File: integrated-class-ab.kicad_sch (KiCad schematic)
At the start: 31 parts, among them J1001 LABEL, Q1001 MMBT3904W, U1001 SL9062D, U1002 LT1794

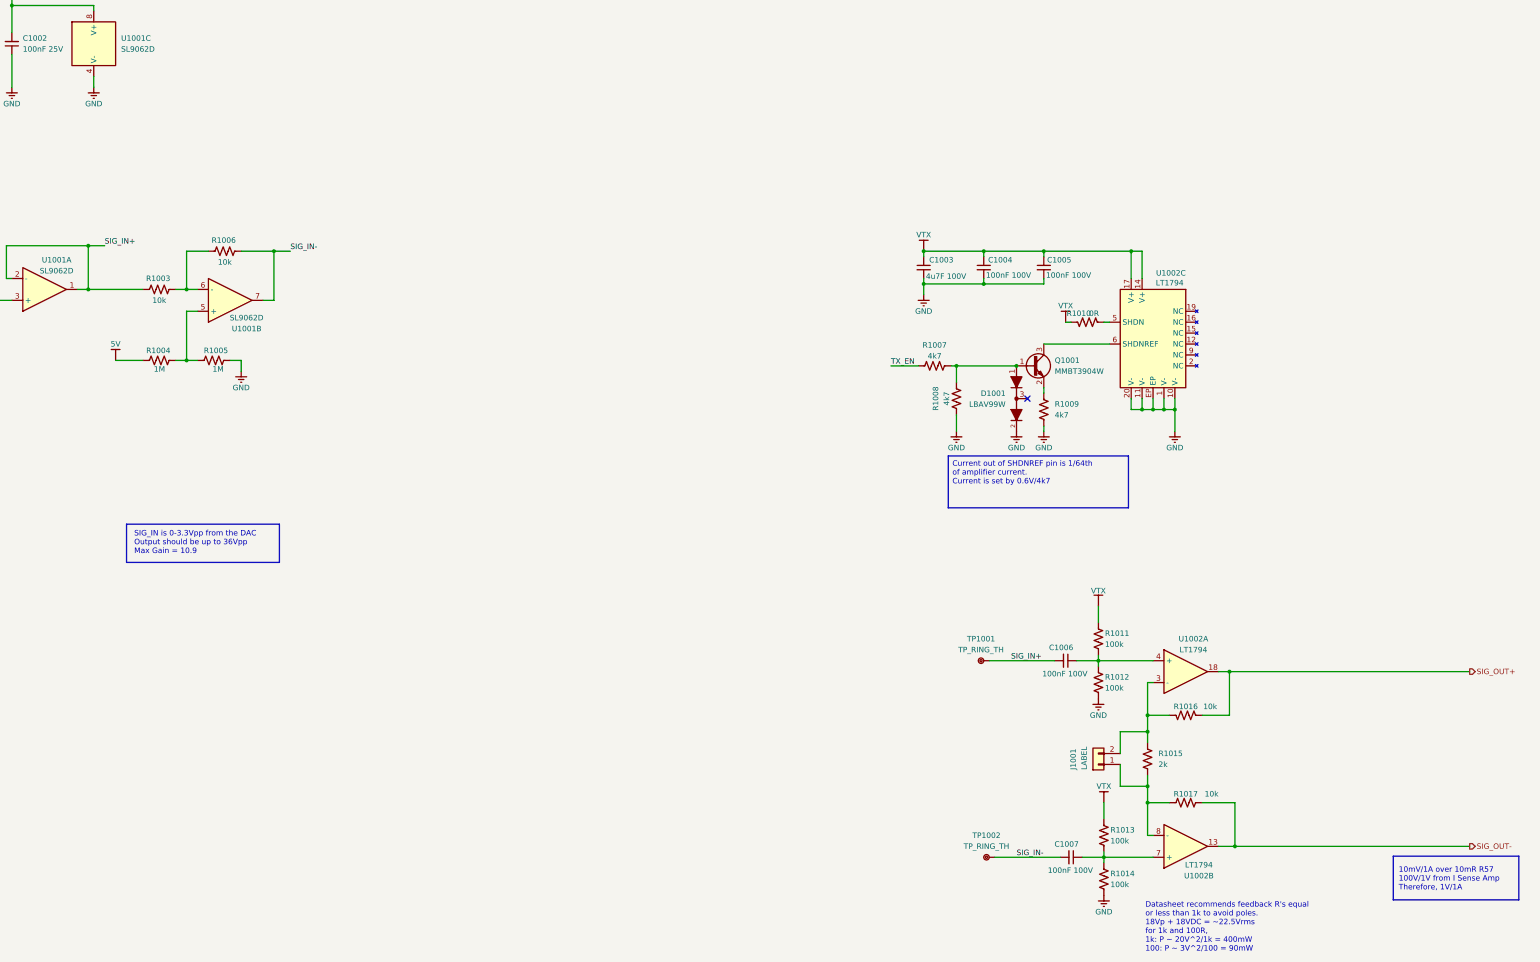
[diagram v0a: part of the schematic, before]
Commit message: more work
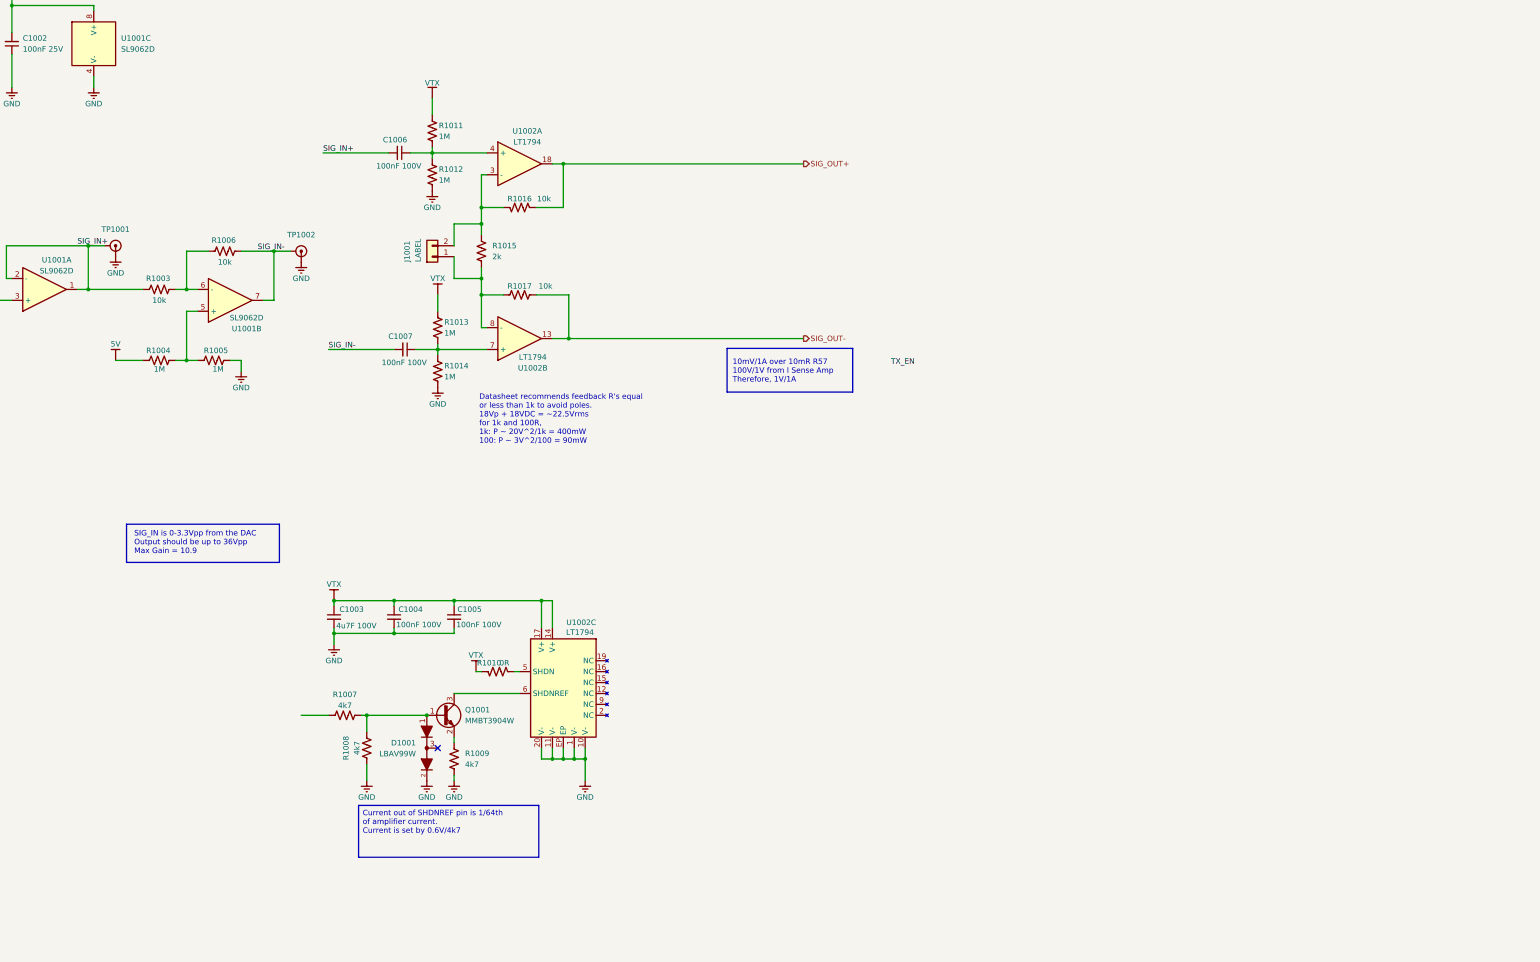
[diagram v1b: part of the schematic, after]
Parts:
- R1011, R1012, R1013, R1014: value 100k -> 1M; footprint BR_Passives:R_0201_0603Metric-minimized -> BR_Passives:C_0402_1005Metric-minimized; symbol BR_Resistors_0201:R_0201_100k -> BR_Resistors_0402:R_0402_1M; BRE Number BRE-001166 -> BRE-000309; JLCPCB Part Num C106224 -> C144787; Manufacturer Part Num RC0201FR-07100KL -> AC0402FR-071ML; Supplier Part Num 1 311-10.0KMCT-ND -> YAG3450CT-ND; Supplier Part Num 2 603-RC0201FR-0710KL -> 603-AC0402FR-071ML; Supplier Part Num 3 C106225 -> C144787
- TP1001, TP1002: value TP_RING_TH -> value; footprint BR_Connectors:TEST-TH_BD2.54-P1.4_RED -> BR_Virtual_Parts:TP_PROBE_TIP_WITH_GND; symbol BR_Connectors:TP_Ring_PTH -> BR_Virtual_Parts:TP_Probe_Tip_0.8mm_Hole_with_GND; now left out of the parts list
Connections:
- net GND: now also TP1001.1, TP1002.1
- net SIG_IN+: now also TP1001.2 (GND); no longer TP1001.1
- net SIG_IN-: now also TP1002.2 (GND); no longer TP1002.1
- net TX_EN: no longer R1007.1
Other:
- moved on the sheet: C1003, C1004, C1005, C1006, C1007, D1001, J1001, Q1001, R1007, R1008, R1009, R1010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
